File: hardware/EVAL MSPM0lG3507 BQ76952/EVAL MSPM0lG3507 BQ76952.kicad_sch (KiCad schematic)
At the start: 68 parts, among them J1 Conn_01x09_Socket, J10 Screw_Terminal_01x02, J11 Screw_Terminal_01x02, J12 Screw_Terminal_01x02, J13 Screw_Terminal_01x02, J14 Screw_Terminal_01x02, J17 Conn_02x02_Odd_Even, J2 Conn_02x05_Odd_Even, J3 Conn_01x04_Pin, J4 Screw_Terminal_01x02, J5 Conn_01x09_Socket, J6 Conn_01x02_Pin, J7 Screw_Terminal_01x02, J8 Screw_Terminal_01x02, J9 Screw_Terminal_01x02, Q6 2N7002, SW1 SW_Push, SW2 SW_Push, U2 MCU-MSM0G3507SPM, U6 TPD4E05U06DQA, U7 TPD4E05U06DQA

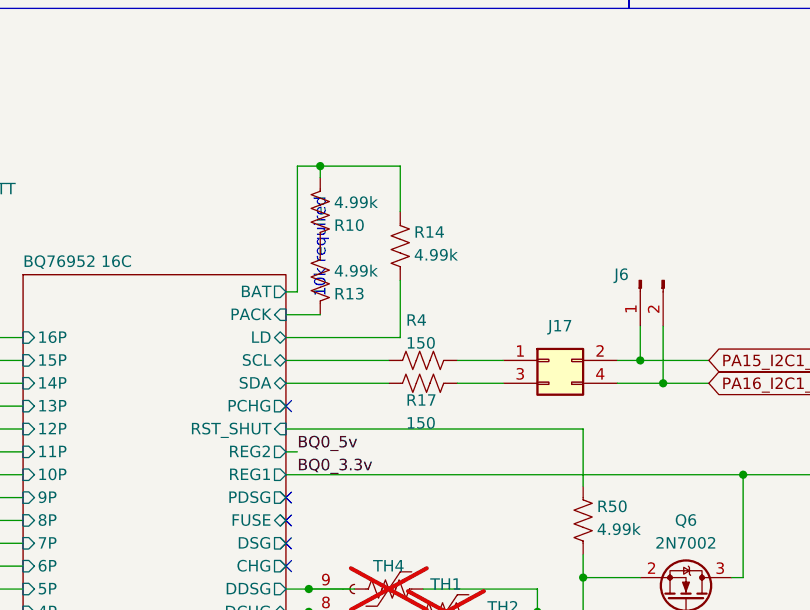
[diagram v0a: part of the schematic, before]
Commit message: bluhhh
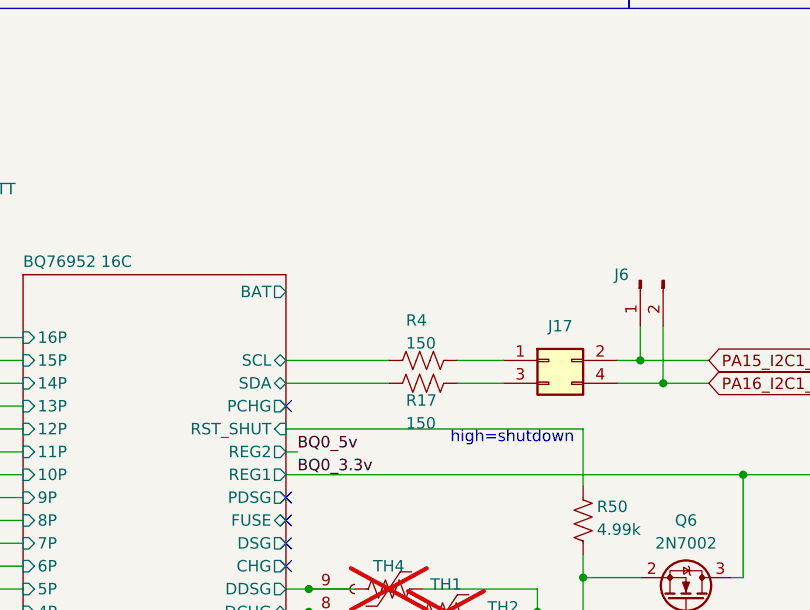
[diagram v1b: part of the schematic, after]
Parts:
- removed R10, R13, R14: 4.99k, Resistor_SMD:R_1206_3216Metric_Pad1.30x1.75mm_HandSolder, symbol Device:R_US
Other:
- sheet BQ76952 16C ports: added none; removed LD, PACK
- note added: "high=shutdown"
- note removed: "10k required"

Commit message: d
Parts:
- J1, J17, J3, J5, J6: mouser (none) -> https://www.mouser.com/ProductDetail/3M-Electronic-Solution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
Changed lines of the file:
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@@
 			)
 		)
+		(property "mouser" "https://www.mouser.com/ProductDetail/3M-Electronic-Solutions-Division/929400-01-07-RK?qs=8Li5tweT5mxAnRwvBSG7wg%3D%3D&mgh=1&utm_id=22693461723&utm_source=google&utm_medium=cpc&utm_marketing_tactic=amercorp&gad_source=1&gad_campaignid=22699465430&gclid=Cj0KCQjw0Y3HBhCxARIsAN7931V3Q9lNZD5h4uJjA3G07-TRSv1KPKk1_9nCCKxyCRbpuWAP8GWV0v4aAg3GEALw_wcB"
+			(at 123.19 127 90)
+			(effects
+				(font
+					(size 1.27 1.27)
+				)
+				(hide yes)
+			)
+		)
 		(pin "1"
 		)
@@
 			)
 		)
+		(property "mouser" "https://www.mouser.com/ProductDetail/3M-Electronic-Solutions-Division/929400-01-07-RK?qs=8Li5tweT5mxAnRwvBSG7wg%3D%3D&mgh=1&utm_id=22693461723&utm_source=google&utm_medium=cpc&utm_marketing_tactic=amercorp&gad_source=1&gad_campaignid=22699465430&gclid=Cj0KCQjw0Y3HBhCxARIsAN7931V3Q9lNZD5h4uJjA3G07-TRSv1KPKk1_9nCCKxyCRbpuWAP8GWV0v4aAg3GEALw_wcB"
+			(at 163.83 83.82 0)
+			(effects
+				(font
+					(size 1.27 1.27)
+				)
+				(hide yes)
+			)
+		)
 		(pin "4"
 		)
@@
 			)
 		)
+		(property "mouser" "https://www.mouser.com/ProductDetail/3M-Electronic-Solutions-Division/929400-01-07-RK?qs=8Li5tweT5mxAnRwvBSG7wg%3D%3D&mgh=1&utm_id=22693461723&utm_source=google&utm_medium=cpc&utm_marketing_tactic=amercorp&gad_source=1&gad_campaignid=22699465430&gclid=Cj0KCQjw0Y3HBhCxARIsAN7931V3Q9lNZD5h4uJjA3G07-TRSv1KPKk1_9nCCKxyCRbpuWAP8GWV0v4aAg3GEALw_wcB"
+			(at 24.13 59.69 0)
+			(effects
+				(font
+					(size 1.27 1.27)
+				)
+				(hide yes)
+			)
+		)
 		(pin "4"
 		)
@@
 			)
 		)
+		(property "mouser" "https://www.mouser.com/ProductDetail/3M-Electronic-Solutions-Division/929400-01-07-RK?qs=8Li5tweT5mxAnRwvBSG7wg%3D%3D&mgh=1&utm_id=22693461723&utm_source=google&utm_medium=cpc&utm_marketing_tactic=amercorp&gad_source=1&gad_campaignid=22699465430&gclid=Cj0KCQjw0Y3HBhCxARIsAN7931V3Q9lNZD5h4uJjA3G07-TRSv1KPKk1_9nCCKxyCRbpuWAP8GWV0v4aAg3GEALw_wcB"
+			(at 91.44 171.45 0)
+			(effects
+				(font
+					(size 1.27 1.27)
+				)
+				(hide yes)
+			)
+		)
 		(pin "4"
 		)
@@
 			(at 113.03 135.89 0)
 			(effects
+				(font
+					(size 1.27 1.27)
+				)
+				(hide yes)
+			)
+		)
+		(property "mouser" "https://www.mouser.com/ProductDetail/3M-Electronic-Solutions-Division/929400-01-07-RK?qs=8Li5tweT5mxAnRwvBSG7wg%3D%3D&mgh=1&utm_id=22693461723&utm_source=google&utm_medium=cpc&utm_marketing_tactic=amercorp&gad_source=1&gad_campaignid=22699465430&gclid=Cj0KCQjw0Y3HBhCxARIsAN7931V3Q9lNZD5h4uJjA3G07-TRSv1KPKk1_9nCCKxyCRbpuWAP8GWV0v4aAg3GEALw_wcB"
+			(at 113.03 135.89 0)
+			(effects

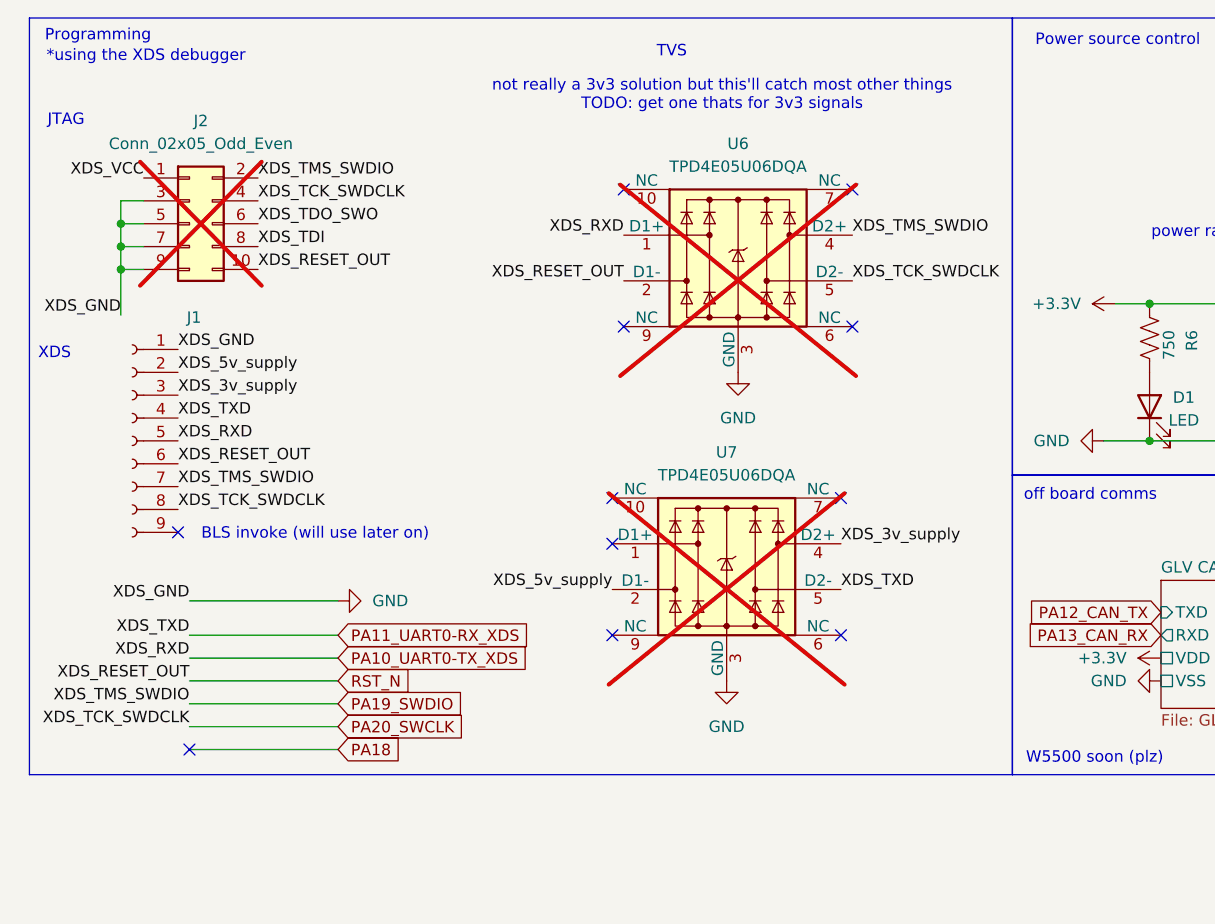
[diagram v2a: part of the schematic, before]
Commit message: ac;lkacnl;
acea;kca
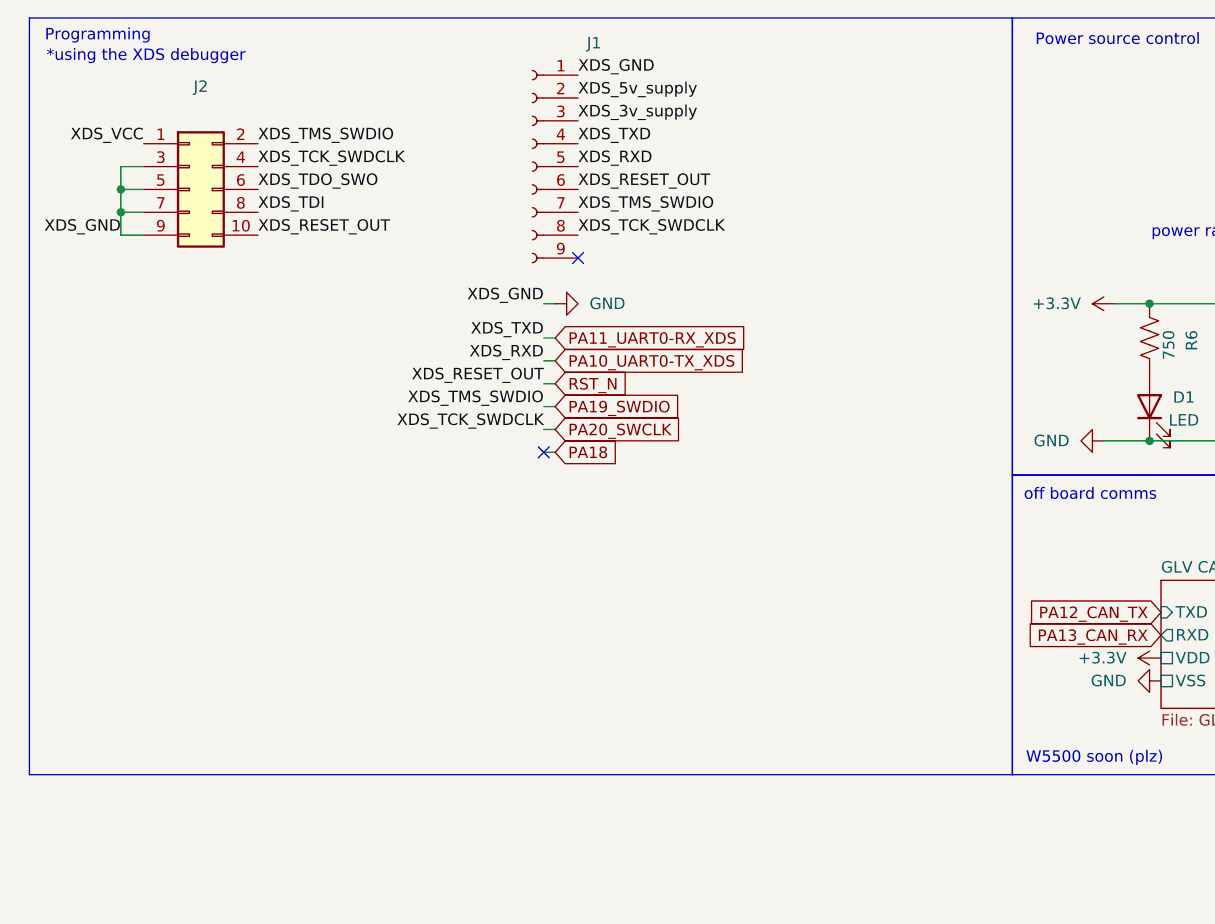
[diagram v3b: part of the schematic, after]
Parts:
- removed U6, U7: TPD4E05U06DQA, Package_SON:USON-10_2.5x1.0mm_P0.5mm, symbol Power_Protection:TPD4E05U06DQA
- J2: now fitted; now in the parts list
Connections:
- no-connect marks 60 -> 51
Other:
- note removed: "BLS invoke (will use later on)"
- note removed: "JTAG"
- note removed: "TVS"
- note removed: "XDS"
- note removed: "not really a 3v3 solution but this'll catch most other things TODO: get one thats for 3v3 signals"
- moved on the sheet: J1
